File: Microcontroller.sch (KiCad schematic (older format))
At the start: 40 parts, among them CN2 CONN_RCPT_USB2.0_MINI_B_SMD_R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, M1 2N7002BK, M2 2N7002BK, Q10 2N7002BK, U2 STM32L476RGLQFP64, X1 ABM3B-16.000MHZ

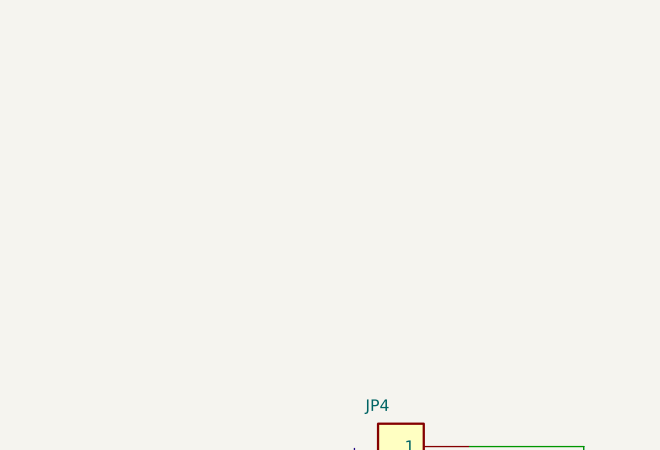
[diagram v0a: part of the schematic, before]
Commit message: Update Microcontroller.sch
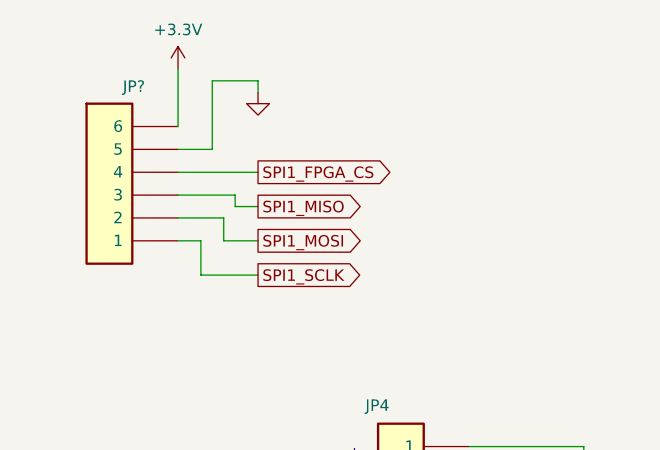
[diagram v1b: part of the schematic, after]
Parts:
- added JP?: Pin_Header,_1x6-Way,_2.54mm_Pitch, symbol OpenVent:Pin_Header,_1x6-Way,_2.54mm_Pitch
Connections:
- wire segments 183 -> 198
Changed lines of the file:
@@
 Wire Wire Line
 	6350 1900 6550 1900
+$Comp
+L OpenVent:Pin_Header,_1x6-Way,_2.54mm_Pitch JP?
+U 1 1 60546722
+P 1100 1000
+F 0 "JP?" H 1293 825 50  0000 C CNN
+F 1 "Pin_Header,_1x6-Way,_2.54mm_Pitch" H 1300 1500 50  0001 C CNN
+F 2 "" H 1300 1500 50  0001 C CNN
+F 3 "" H 1300 1500 50  0001 C CNN
+	1    1100 1000
+	-1   0    0    1
+$EndComp
+$Comp
+L OpenVent:+3.3V #PWR?
+U 1 1 60547AA4
+P 1100 750
+F 0 "#PWR?" H 1100 600 50  0001 C CNN
+F 1 "+3.3V" H 1100 923 50  0000 C CNN
+F 2 "" H 1100 750 50  0001 C CNN
+F 3 "" H 1100 750 50  0001 C CNN
+	1    1100 750
+	1    0    0    -1
+$EndComp
+$Comp
+L OpenVent:GND #PWR?
+U 1 1 60548A69
+P 1450 850
+F 0 "#PWR?" H 1450 600 50  0001 C CNN
+F 1 "GND" H 1450 700 50  0001 C CNN
+F 2 "" H 1450 850 50  0001 C CNN
+F 3 "" H 1450 850 50  0001 C CNN
+	1    1450 850
+	1    0    0    -1
+$EndComp
+Wire Wire Line
+	1100 1000 1100 750
+Wire Wire Line
+	1100 1100 1250 1100
+Wire Wire Line
+	1450 800  1450 850
+Text GLabel 1450 1200 2    50   Output ~ 0
+SPI1_FPGA_CS
+Text GLabel 1450 1350 2    50   Output ~ 0
+SPI1_MISO
+Text GLabel 1450 1500 2    50   Output ~ 0
+SPI1_MOSI
+Text GLabel 1450 1650 2    50   Output ~ 0
+SPI1_SCLK
+Wire Wire Line
+	1250 1100 1250 800
+Wire Wire Line
+	1250 800  1450 800
+Wire Wire Line
+	1100 1200 1450 1200
+Wire Wire Line
+	1100 1300 1350 1300
+Wire Wire Line
+	1350 1300 1350 1350
+Wire Wire Line
+	1350 1350 1450 1350
+Wire Wire Line
+	1100 1400 1300 1400
+Wire Wire Line
+	1300 1400 1300 1500
+Wire Wire Line
+	1300 1500 1450 1500
+Wire Wire Line
+	1100 1500 1200 1500
+Wire Wire Line
+	1200 1500 1200 1650
+Wire Wire Line
+	1200 1650 1450 1650
 $EndSCHEMATC

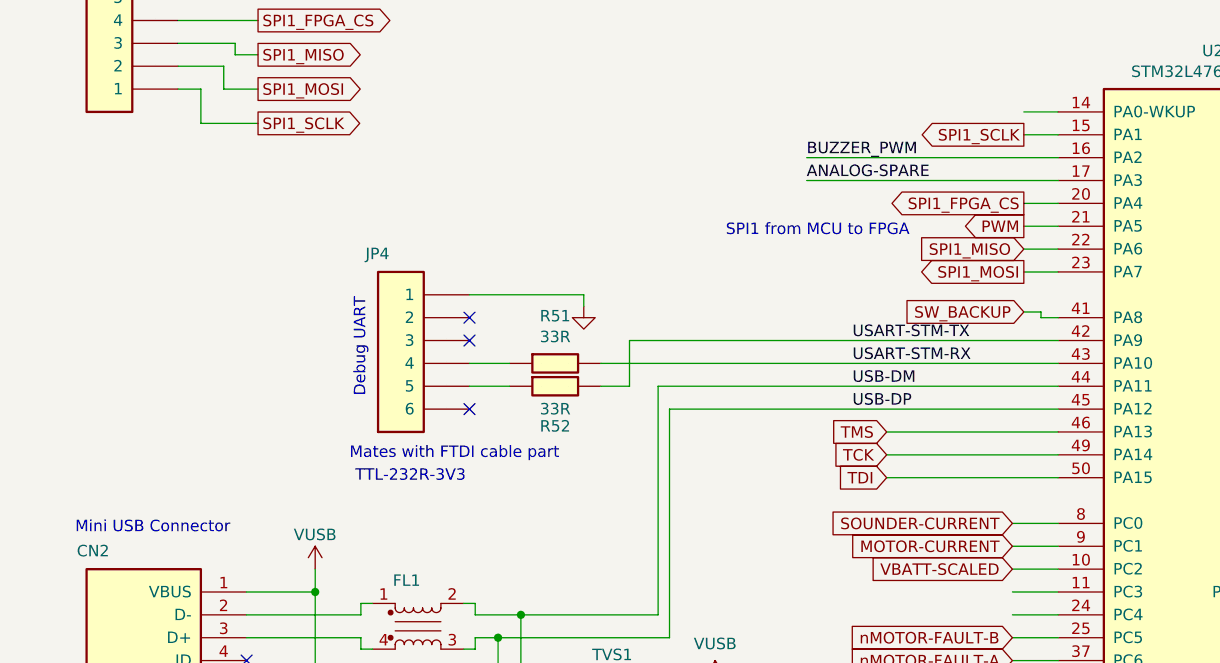
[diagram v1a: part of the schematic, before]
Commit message: Update Microcontroller.sch
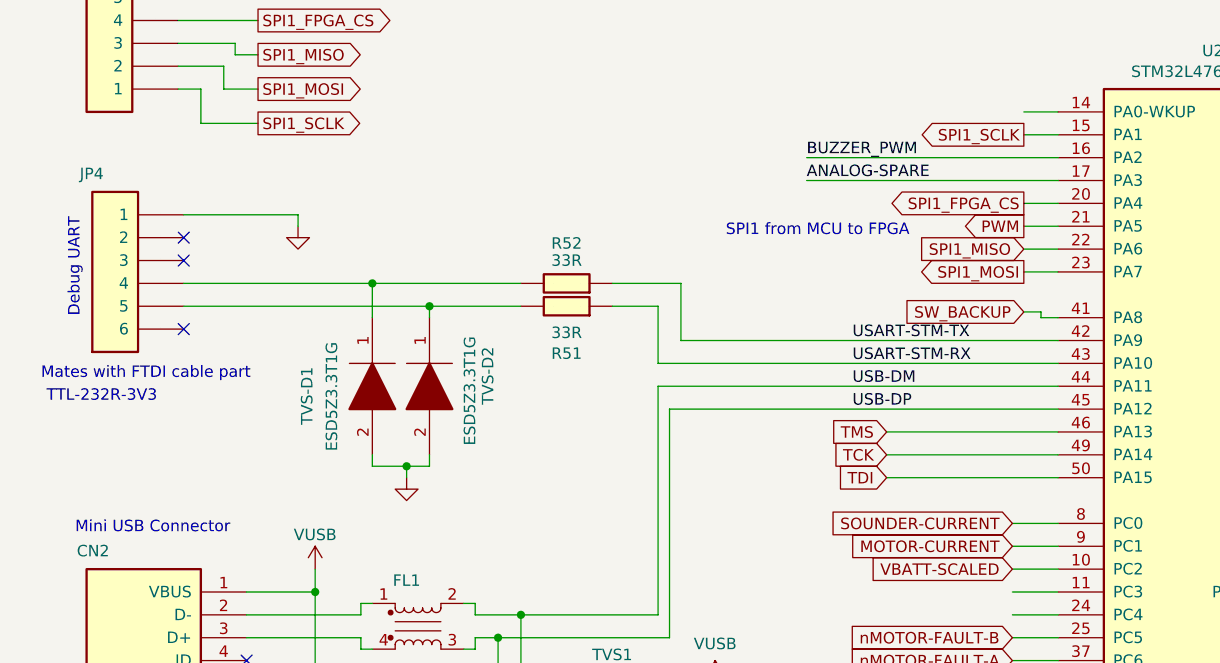
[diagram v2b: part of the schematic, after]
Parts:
- added TVS-D1, TVS-D2: ESD5Z3.3T1G, SODFL1608X70N, symbol OpenVent:ESD5Z3.3T1G
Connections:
- wire segments 198 -> 209
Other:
- moved on the sheet: JP4, R51, R52
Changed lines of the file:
@@
 Comment4 ""
 $EndDescr
-Text Notes 1925 2850 1    50   ~ 0
+Text Notes 675  2500 1    50   ~ 0
 Debug UART
-Text Notes 1850 3125 0    50   ~ 0
+Text Notes 500  2775 0    50   ~ 0
 Mates with FTDI cable part
 Text GLabel 6550 2900 2    50   Output ~ 0
@@
 L OpenVent:GND #GND_07
 U 1 1 5F8DD179
-P 2875 2450
-F 0 "#GND_07" H 2875 2450 20  0001 C CNN
-F 1 "GND" H 2875 2380 50  0001 C CNN
-F 2 "" H 2875 2450 70  0001 C CNN
-F 3 "" H 2875 2450 70  0001 C CNN
-	1    2875 2450
+P 1625 2100
+F 0 "#GND_07" H 1625 2100 20  0001 C CNN
+F 1 "GND" H 1625 2030 50  0001 C CNN
+F 2 "" H 1625 2100 70  0001 C CNN
+F 3 "" H 1625 2100 70  0001 C CNN
+	1    1625 2100
 	1    0    0    -1
 $EndComp
 Text GLabel 4750 3600 0    50   Input ~ 0
 VBATT-SCALED
-NoConn ~ 2375 2600
+NoConn ~ 1125 2250
 Text GLabel 4750 3500 0    50   Input ~ 0
 MOTOR-CURRENT
@@
 Text Label 4050 2700 0    50   ~ 0
 USART-STM-RX
-NoConn ~ 2375 2500
-NoConn ~ 2375 2900
+NoConn ~ 1125 2150
+NoConn ~ 1125 2550
 $Comp
 L OpenVent:3V3 #3V3_03
@@
 	1    0    0    -1
 $EndComp
-Text Notes 1875 3225 0    50   ~ 0
+Text Notes 525  2875 0    50   ~ 0
 TTL-232R-3V3
 Text GLabel 4750 4000 0    50   Input ~ 0
@@
 	1700 4050 1700 3700
 Wire Wire Line
-	4950 2600 3075 2600
-Wire Wire Line
-	2375 2700 2550 2700
-Wire Wire Line
-	2875 2400 2375 2400
-Wire Wire Line
-	2875 2450 2875 2400
+	1625 2050 1125 2050
+Wire Wire Line
+	1625 2100 1625 2050
 Wire Wire Line
 	4975 6825 4325 6825
@@
 L OpenVent:Pin_Header,_1x6-Way,_2.54mm_Pitch JP4
 U 1 1 5F8DD14A
-P 2375 2900
-F 0 "JP4" H 2725 3550 50  0000 L BNN
-F 1 "Pin_Header,_1x6-Way,_2.54mm_Pitch" H 2375 2900 50  0001 C CNN
-F 2 "Connector_PinHeader_2.54mm:PinHeader_1x06_P2.54mm_Vertical" H 2375 2900 50  0001 C CNN
-F 3 "" H 2375 2900 50  0001 C CNN
-	1    2375 2900
+P 1125 2550
+F 0 "JP4" H 1475 3200 50  0000 L BNN
+F 1 "Pin_Header,_1x6-Way,_2.54mm_Pitch" H 1125 2550 50  0001 C CNN
+F 2 "Connector_PinHeader_2.54mm:PinHeader_1x06_P2.54mm_Vertical" H 1125 2550 50  0001 C CNN
+F 3 "" H 1125 2550 50  0001 C CNN
+	1    1125 2550
 	-1   0    0    -1
 $EndComp
@@
 L OpenVent:33R_Chip_Resistor,_1%,_0.1W R51
 U 1 1 5FF35864
-P 2650 2600
-F 0 "R51" H 2750 2707 50  0000 C CNN
-F 1 "33R_Chip_Resistor,_1%,_0.1W" H 2300 2950 50  0001 C CNN
-F 2 "" H 2850 2600 50  0001 C CNN
-F 3 "" H 2650 2600 50  0001 C CNN
-F 4 "33R" H 2750 2616 50  0000 C CNN "Val"
-F 5 "1%" H 3200 2600 50  0001 C CNN "Tolerance"
-F 6 "0.1W" H 2650 2600 50  0001 C CNN "Watt"
-	1    2650 2600
-	1    0    0    -1
+P 2900 2550
+F 0 "R51" H 3000 2657 50  0000 C CNN
+F 1 "33R_Chip_Resistor,_1%,_0.1W" H 2550 2900 50  0001 C CNN
+F 2 "" H 3100 2550 50  0001 C CNN
+F 3 "" H 2900 2550 50  0001 C CNN
+F 4 "33R" H 3000 2566 50  0000 C CNN "Val"
+F 5 "1%" H 3450 2550 50  0001 C CNN "Tolerance"
+F 6 "0.1W" H 2900 2550 50  0001 C CNN "Watt"
+	1    2900 2550
+	-1   0    0    1
 $EndComp
 $Comp
 L OpenVent:33R_Chip_Resistor,_1%,_0.1W R52
 U 1 1 5FF35DAD
-P 2650 2700
-F 0 "R52" H 2750 2425 50  0000 C CNN
-F 1 "33R_Chip_Resistor,_1%,_0.1W" H 2300 3050 50  0001 C CNN
-F 2 "" H 2850 2700 50  0001 C CNN
-F 3 "" H 2650 2700 50  0001 C CNN
-F 4 "33R" H 2750 2500 50  0000 C CNN "Val"
-F 5 "1%" H 3200 2700 50  0001 C CNN "Tolerance"
-F 6 "0.1W" H 2650 2700 50  0001 C CNN "Watt"
-	1    2650 2700
-	1    0    0    -1
-$EndComp
-Wire Wire Line
-	2550 2800 2375 2800
-Wire Wire Line
-	3075 2600 3075 2800
-Wire Wire Line
-	2950 2800 3075 2800
-Wire Wire Line
-	2950 2700 4950 2700
+P 2900 2450
+F 0 "R52" H 3000 2175 50  0000 C CNN
+F 1 "33R_Chip_Resistor,_1%,_0.1W" H 2550 2800 50  0001 C CNN
+F 2 "" H 3100 2450 50  0001 C CNN
+F 3 "" H 2900 2450 50  0001 C CNN
+F 4 "33R" H 3000 2250 50  0000 C CNN "Val"
+F 5 "1%" H 3450 2450 50  0001 C CNN "Tolerance"
+F 6 "0.1W" H 2900 2450 50  0001 C CNN "Watt"
+	1    2900 2450
+	-1   0    0    1
+$EndComp
 Wire Wire Line
 	6975 6225 6975 6175
@@
 Wire Wire Line
 	1200 1650 1450 1650
+$Comp
+L OpenVent:ESD5Z3.3T1G TVS-D2
+U 1 1 605B29D3
+P 2200 2500
+F 0 "TVS-D2" H 2454 2756 50  0000 C CNN
+F 1 "ESD5Z3.3T1G" H 2520 2677 50  0000 C CNN
+F 2 "SODFL1608X70N" H 2650 2500 50  0001 L CNN
+F 3 "http://www.onsemi.com/pub/Collateral/ESD5Z2.5T1-D.PDF" H 2650 2400 50  0001 L CNN
+F 4 "TVS Diode Uni-Direct. 240W 3.3V SOD-523 ON Semiconductor ESD5Z3.3T1G Uni-Directional TVS Diode, 200W peak, 2-Pin SOD-523" H 2650 2300 50  0001 L CNN "Description"
+F 5 "0.7" H 2650 2200 50  0001 L CNN "Height"
+F 6 "ON Semiconductor" H 2650 2100 50  0001 L CNN "Manufacturer_Name"
+F 7 "ESD5Z3.3T1G" H 2650 2000 50  0001 L CNN "Manufacturer_Part_Number"
+F 8 "863-ESD5Z3.3T1G" H 2650 1900 50  0001 L CNN "Mouser Part Number"
+F 9 "https://www.mouser.co.uk/ProductDetail/ON-Semiconductor/ESD5Z33T1G/?qs=OSf9jACorvaH3Y8oRWEcuQ%3D%3D" H 2650 1800 50  0001 L CNN "Mouser Price/Stock"
+F 10 "ESD5Z3.3T1G" H 2650 1700 50  0001 L CNN "Arrow Part Number"
+F 11 "https://www.arrow.com/en/products/esd5z3.3t1g/on-semiconductor" H 2650 1600 50  0001 L CNN "Arrow Price/Stock"
+	1    2200 2500
+	0    1    1    0
+$EndComp
+$Comp
+L OpenVent:ESD5Z3.3T1G TVS-D1
+U 1 1 605B4E90
+P 1950 2500
+F 0 "TVS-D1" H 2165 2244 50  0000 L TNN
+F 1 "ESD5Z3.3T1G" H 2295 2323 50  0000 C CNN
+F 2 "SODFL1608X70N" H 2400 2500 50  0001 L CNN
+F 3 "http://www.onsemi.com/pub/Collateral/ESD5Z2.5T1-D.PDF" H 2400 2400 50  0001 L CNN
+F 4 "TVS Diode Uni-Direct. 240W 3.3V SOD-523 ON Semiconductor ESD5Z3.3T1G Uni-Directional TVS Diode, 200W peak, 2-Pin SOD-523" H 2400 2300 50  0001 L CNN "Description"
+F 5 "0.7" H 2400 2200 50  0001 L CNN "Height"
+F 6 "ON Semiconductor" H 2400 2100 50  0001 L CNN "Manufacturer_Name"
+F 7 "ESD5Z3.3T1G" H 2400 2000 50  0001 L CNN "Manufacturer_Part_Number"
+F 8 "863-ESD5Z3.3T1G" H 2400 1900 50  0001 L CNN "Mouser Part Number"
+F 9 "https://www.mouser.co.uk/ProductDetail/ON-Semiconductor/ESD5Z33T1G/?qs=OSf9jACorvaH3Y8oRWEcuQ%3D%3D" H 2400 1800 50  0001 L CNN "Mouser Price/Stock"
+F 10 "ESD5Z3.3T1G" H 2400 1700 50  0001 L CNN "Arrow Part Number"
+F 11 "https://www.arrow.com/en/products/esd5z3.3t1g/on-semiconductor" H 2400 1600 50  0001 L CNN "Arrow Price/Stock"
+	1    1950 2500
+	0    1    1    0
+$EndComp
+Wire Wire Line
+	1125 2350 1950 2350
+Wire Wire Line
+	1125 2450 2200 2450
+Wire Wire Line
+	2200 2500 2200 2450
+Connection ~ 2200 2450
+Wire Wire Line
+	1950 2500 1950 2350
+Connection ~ 1950 2350
+Wire Wire Line
+	1950 3100 1950 3150
+Wire Wire Line
+	1950 3150 2100 3150
+Wire Wire Line
+	2200 3150 2200 3100
+$Comp
+L OpenVent:GND #PWR?
+U 1 1 606192F5
+P 2100 3200
+F 0 "#PWR?" H 2100 2950 50  0001 C CNN
+F 1 "GND" H 2100 3050 50  0001 C CNN
+F 2 "" H 2100 3200 50  0001 C CNN
+F 3 "" H 2100 3200 50  0001 C CNN
+	1    2100 3200
+	1    0    0    -1
+$EndComp
+Wire Wire Line
+	2100 3200 2100 3150
+Connection ~ 2100 3150
+Wire Wire Line
+	2100 3150 2200 3150
+Wire Wire Line
+	4950 2600 3300 2600
+Wire Wire Line
+	3300 2350 3300 2600
+Wire Wire Line
+	3000 2350 3300 2350
+Wire Wire Line
+	3200 2450 3200 2700
+Wire Wire Line
+	3000 2450 3200 2450
+Wire Wire Line
+	3200 2700 4950 2700
+Wire Wire Line
+	1950 2350 2600 2350
+Wire Wire Line
+	2200 2450 2600 2450
 $EndSCHEMATC

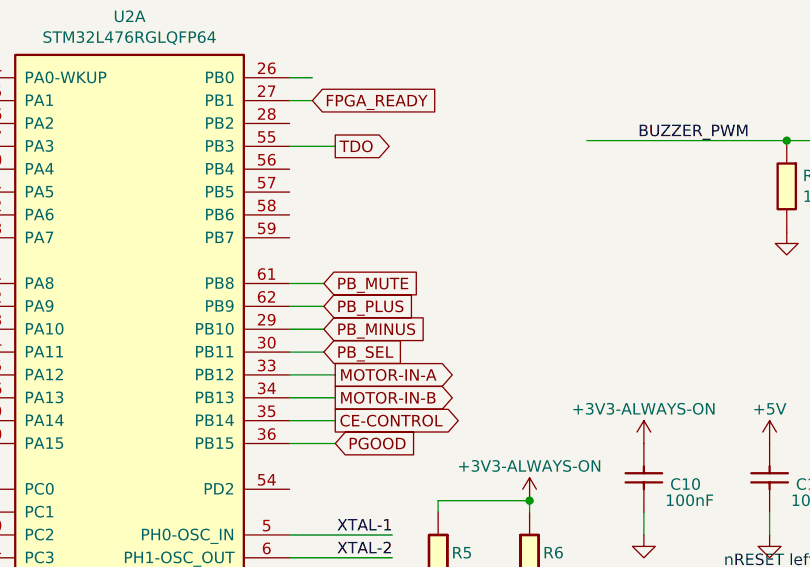
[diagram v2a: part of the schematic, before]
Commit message: Update Microcontroller.sch
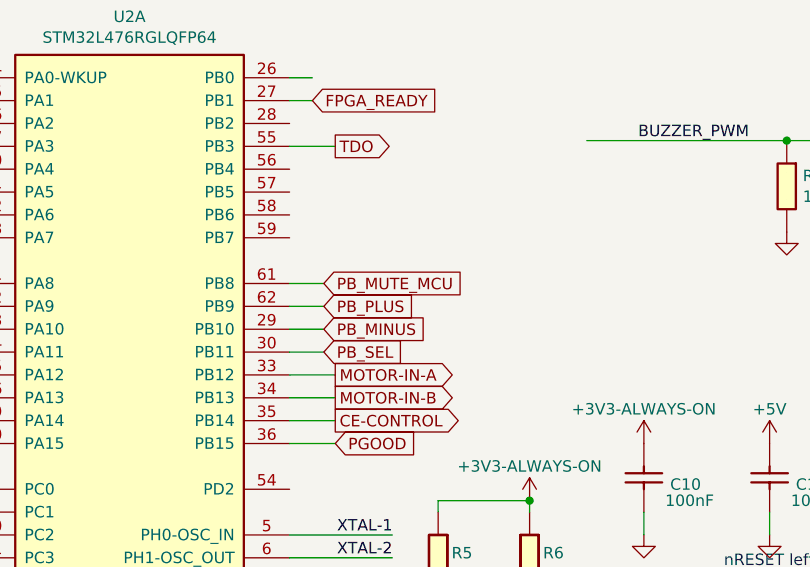
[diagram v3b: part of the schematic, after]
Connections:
- net labels added: PB_MUTE_MCU
- net labels removed: PB_MUTE
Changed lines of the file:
@@
 BUZZER_PWM
 Text GLabel 6500 2500 2    50   Input ~ 0
-PB_MUTE
+PB_MUTE_MCU
 Text GLabel 6500 2600 2    50   Input ~ 0
 PB_PLUS
